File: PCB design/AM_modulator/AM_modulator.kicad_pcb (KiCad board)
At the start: 2 copper layers, 64 x 51.5 mm, 33 parts, among them J1 AudioJack3, J2 Conn_01x02_Female, J3 SMA_CONNECTOR, J4 SMA_CONNECTOR, Q1 MMBT3904, SW1 SW_DIP_x01, SW2 SW_DIP_x01, SW3 SW_DIP_x01, SW4 SW_DIP_x01

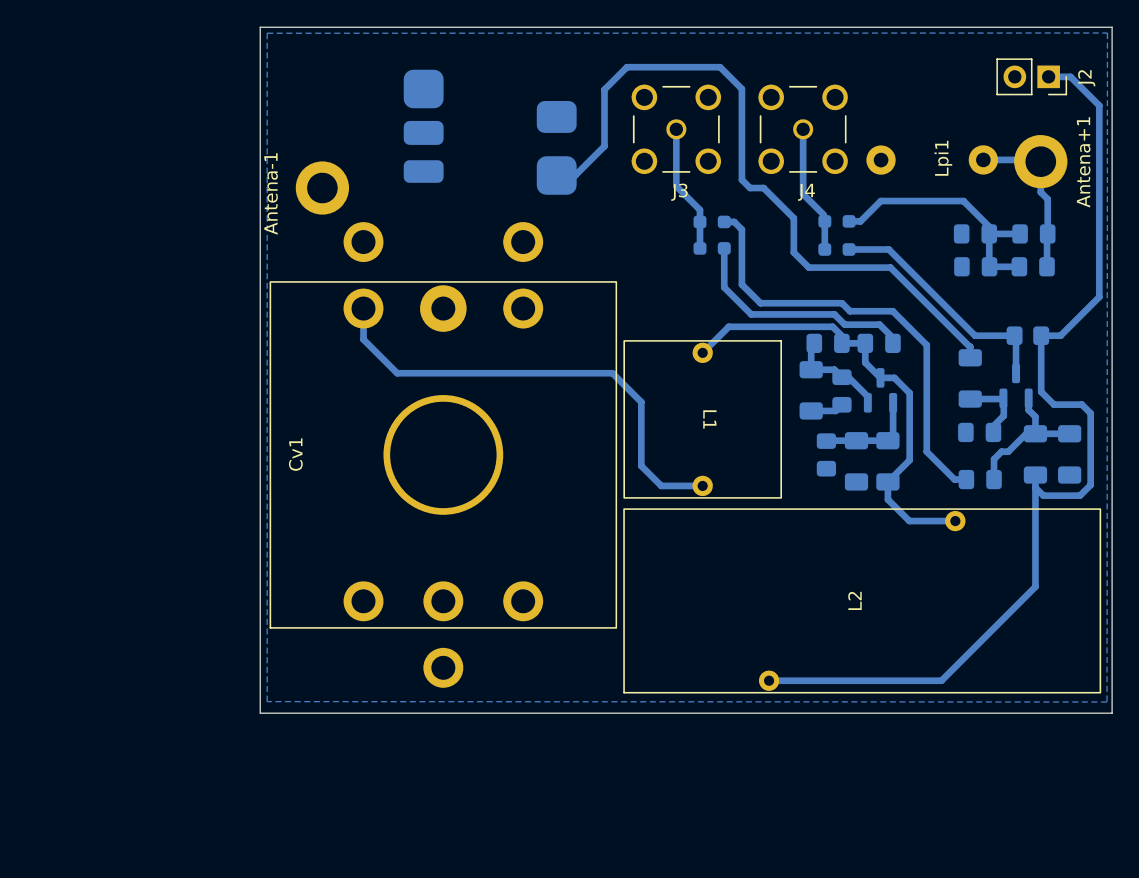
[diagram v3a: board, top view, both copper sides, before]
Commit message: PCB design done
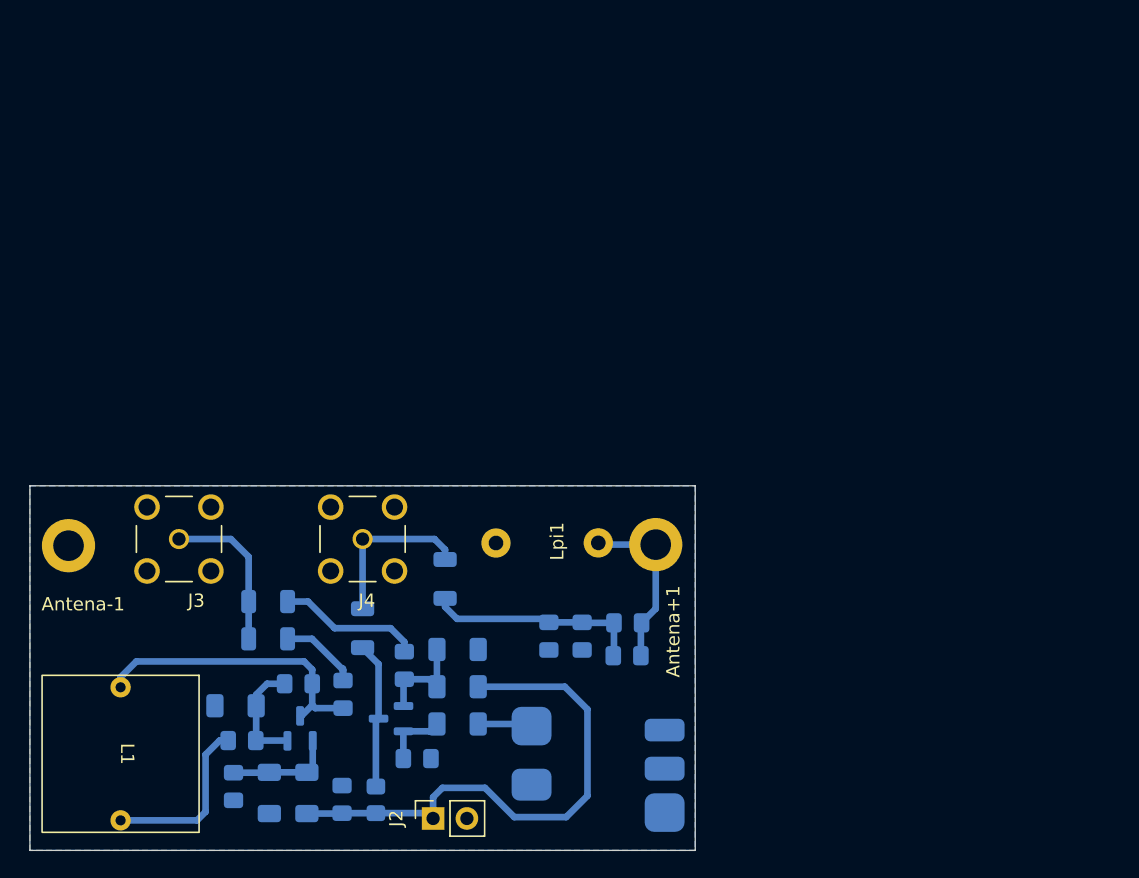
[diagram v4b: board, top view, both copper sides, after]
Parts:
- removed Cv1: 30p, capacitors:variable_cap
- removed L2: 10u, inductors:T-130
- added C5: 100n, Capacitor_SMD:C_0805_2012Metric_Pad1.18x1.45mm_HandSolder, B.Cu at (109.0, 126.7)
- C1: value 1n -> 220p
- C2: value 10n -> 220p
- Cpi1, Cpi11: value C -> 220p
- Cpi2, Cpi21: value C -> 33p
- L1: value 938.16n -> 250n
- Lpi1: value L -> 551.6nH
- R1: value 6.8k -> 10k
- R2: value 3.3k -> 15k
- R3: value 68 -> 470
- SW1, SW2, SW3, SW4: footprint Resistor_SMD:R_0603_1608Metric_Pad0.98x0.95mm_HandSolder -> Resistor_SMD:R_1206_3216Metric
- moved J2 72.4 mm to (115.8, 128.1), turned to 90 degrees
- moved RMc1 60.1 mm to (111.5, 126.7), turned to 90 degrees
- moved QM1 53.2 mm to (112.6, 120.6), turned to 180 degrees
- moved C2 52.2 mm to (101.4, 122.2), turned to 180 degrees
- moved SW2 51.4 mm to (103.4, 111.8)
- moved C3 51.1 mm to (100.8, 125.7)
- moved R2 50.7 mm to (103.5, 126.2)
- moved Q1 50.5 mm to (105.8, 121.3)
- moved L1 50.5 mm to (92.3, 123.2)
- moved R1 50.3 mm to (106.3, 126.2)
- moved R3 49.3 mm to (101.0, 119.6), turned to 180 degrees
- moved CMa1 48.9 mm to (114.6, 123.6), turned to 0 degrees
- moved J3 48.4 mm to (96.7, 107.1)
- moved J1 48.3 mm to (128.2, 124.3), turned to 90 degrees
- moved RMb2 48.3 mm to (117.6, 115.4), turned to 0 degrees
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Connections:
- net /Mixer/Audio renamed /audio
- C2 pad 2: GND -> Net-(C2-Pad2)
- C4 pad 2: Net-(C4-Pad2) -> /SMA_probe/signal_in
- J3 pad 1: /clapp_oscillator/Vout_30MHz_50Ohm -> Net-(SW1-Pad2)
- J4 pad 1: /Mixer/RF -> Net-(SW3-Pad2)
- L1 pad 2: Net-(Cv1-Pad1) -> Net-(C2-Pad2)
- QM1 pad 3: Net-(QM1-Pad3) -> /Mixer/RF
- R1 pad 1: Net-(C1-Pad1) -> +12V
- RMc1 pad 2: Net-(QM1-Pad3) -> /Mixer/RF
- SW1 pad 1: /clapp_oscillator/Vout_30MHz_50Ohm -> /SMA_probe/signal_in
- SW1 pad 2: /Mixer/LO -> Net-(SW1-Pad2)
- SW2 pad 1: /Mixer/RF -> Net-(SW1-Pad2)
- SW2 pad 2: /Antenna/RF_Antenna -> /Mixer/LO
- SW3 pad 1: Net-(C4-Pad2) -> /Mixer/RF
- SW3 pad 2: /clapp_oscillator/Vout_30MHz_50Ohm -> Net-(SW3-Pad2)
- SW4 pad 1: Net-(QM1-Pad3) -> Net-(SW3-Pad2)
- SW4 pad 2: /Mixer/RF -> /Antenna/RF_Antenna
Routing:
- net /audio: track 52.0 -> 4.08 mm
- net Net-(Cv1-Pad1): track 35.2 -> 0.00 mm
- net +12V: track 75.2 -> 40.1 mm
- net /Mixer/LO: track 33.3 -> 10.8 mm
- net Net-(QM1-Pad3): track 18.1 -> 0.00 mm
- net Net-(C4-Pad2): track 17.6 -> 0.00 mm
- net Net-(C2-Pad2): track 0.00 -> 13.1 mm
- net Net-(SW3-Pad2): track 0.00 -> 12.5 mm
- net Net-(SW1-Pad2): track 0.00 -> 12.0 mm
- net Net-(C1-Pad1): track 34.0 -> 22.2 mm
- net /clapp_oscillator/Vout_30MHz_50Ohm: track 9.69 -> 0.00 mm
- net /SMA_probe/signal_in: track 0.00 -> 6.84 mm
- net Net-(CMLO1-Pad1): track 11.2 -> 7.52 mm
- net /Antenna/RF_Antenna: track 19.5 -> 16.3 mm
- net GND: track 2.50 -> 0.00 mm
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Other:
- board size 64 x 51.5 mm -> 50 x 27.4 mm

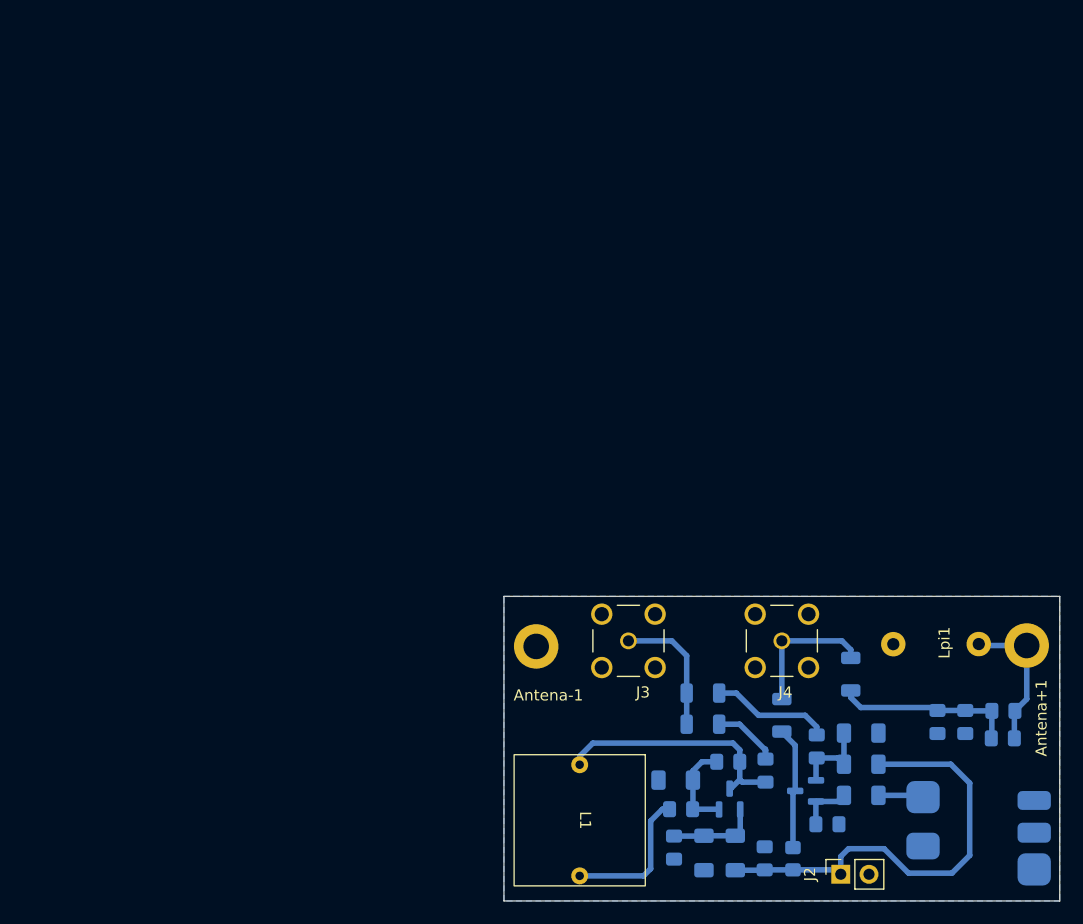
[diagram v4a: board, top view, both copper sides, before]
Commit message: PCB design done
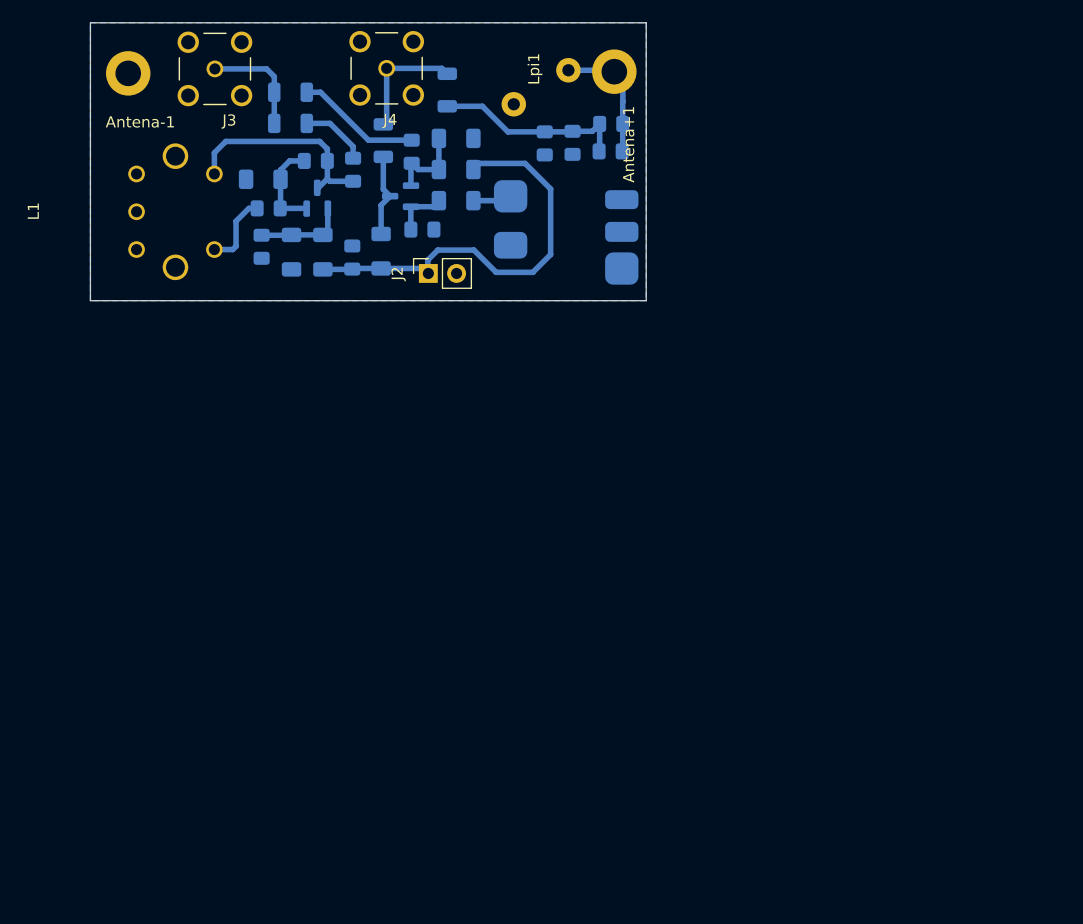
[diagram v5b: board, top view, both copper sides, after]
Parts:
- L1: footprint inductors:air_core_1cm -> inductors:variable_inductor
- RMc1: value 220 -> 240; footprint Resistor_SMD:R_0805_2012Metric_Pad1.20x1.40mm_HandSolder -> Resistor_SMD:R_1206_3216Metric_Pad1.30x1.75mm_HandSolder
- moved RMc1 66.0 mm to (74.5, 72.0)
- moved L1 65.7 mm to (56.0, 68.5), turned to 90 degrees
- moved C5 65.6 mm to (71.9, 72.6)
- moved C2 65.6 mm to (64.3, 68.2)
- moved C4 65.6 mm to (71.9, 64.7)
- moved R1 65.6 mm to (69.2, 72.1)
- moved R2 65.6 mm to (66.4, 72.1)
- moved SW1 65.6 mm to (66.3, 60.5)
- moved SW2 65.6 mm to (66.3, 57.8)
- moved C1 65.6 mm to (68.6, 63.9)
- moved C3 65.6 mm to (63.7, 71.7)
- moved J1 65.6 mm to (91.1, 70.2)
- moved J2 65.6 mm to (78.7, 74.0)
- moved Q1 65.6 mm to (68.7, 67.3)
- moved R3 65.6 mm to (63.9, 65.6)
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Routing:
- net Net-(C2-Pad2): track 13.1 -> 6.70 mm
- net /Mixer/RF: track 11.0 -> 7.53 mm
- net Net-(C1-Pad1): track 22.2 -> 19.1 mm
- net +12V: track 40.1 -> 37.9 mm
- net Net-(J3-Pad1): track 12.0 -> 9.83 mm
- net Net-(J4-Pad1): track 12.5 -> 10.8 mm
- net Net-(Antena+1-Pad1): track 13.2 -> 11.7 mm
- net /Antenna/RF_Antenna: track 16.3 -> 17.5 mm
- net /SMA_probe/signal_in: track 6.84 -> 6.08 mm
- net /audio: track 4.08 -> 3.51 mm
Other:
- board size 50 x 27.4 mm -> 50 x 25 mm
